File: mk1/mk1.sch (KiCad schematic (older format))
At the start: 121 parts, among them U1 STM32F070CBTx

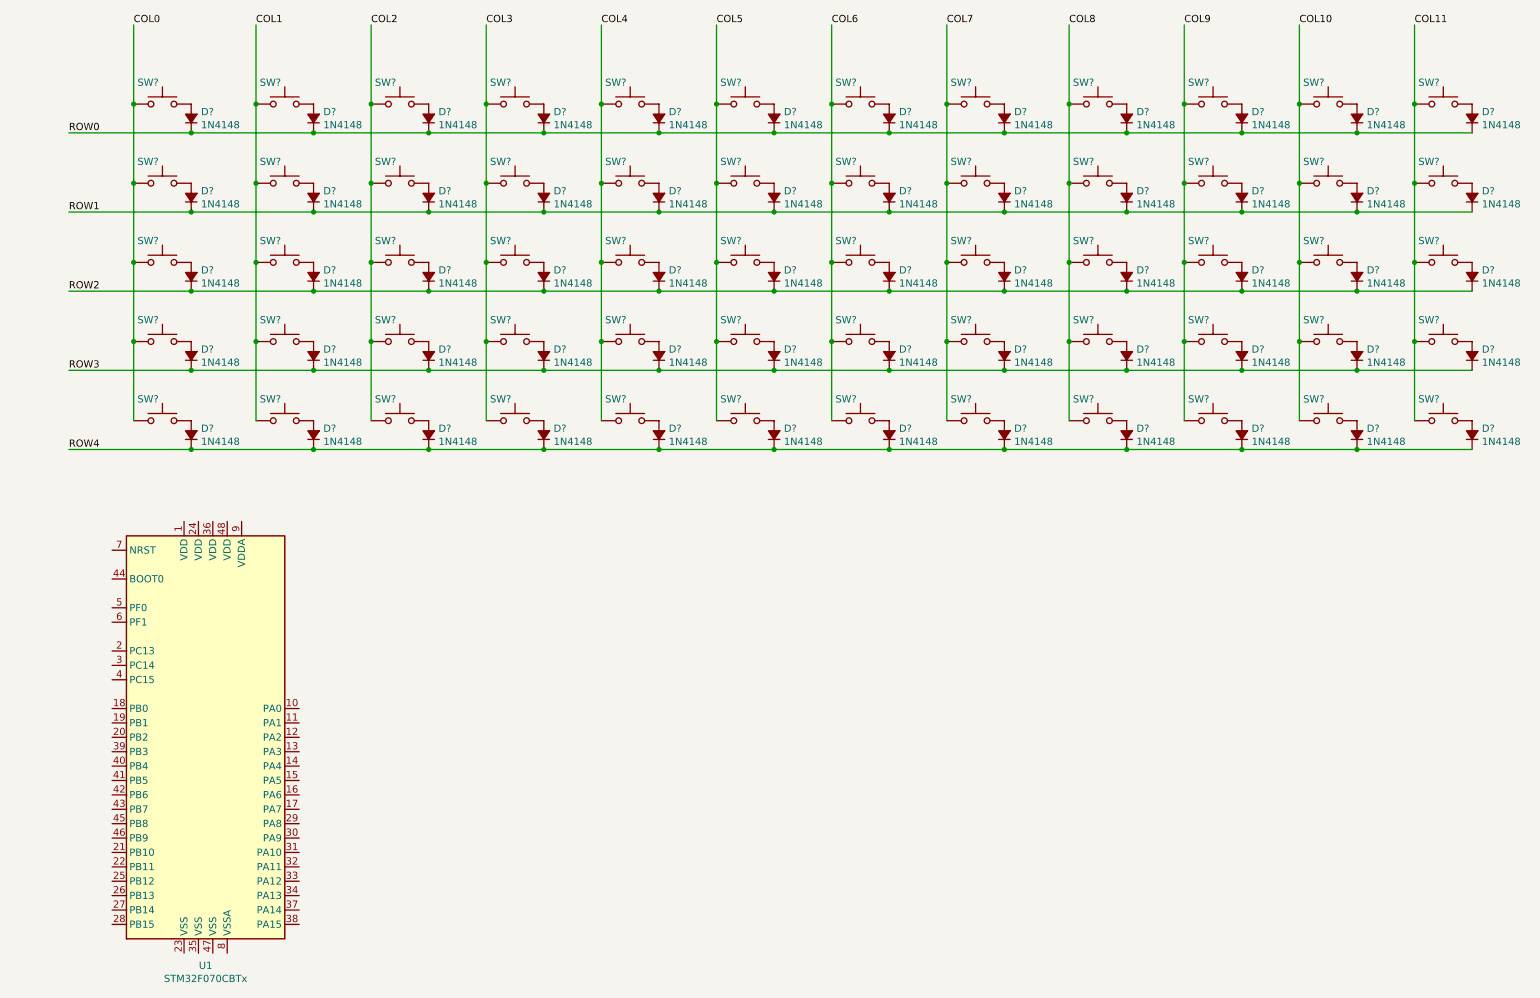
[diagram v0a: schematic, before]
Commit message: using ML switch built i jumper bar
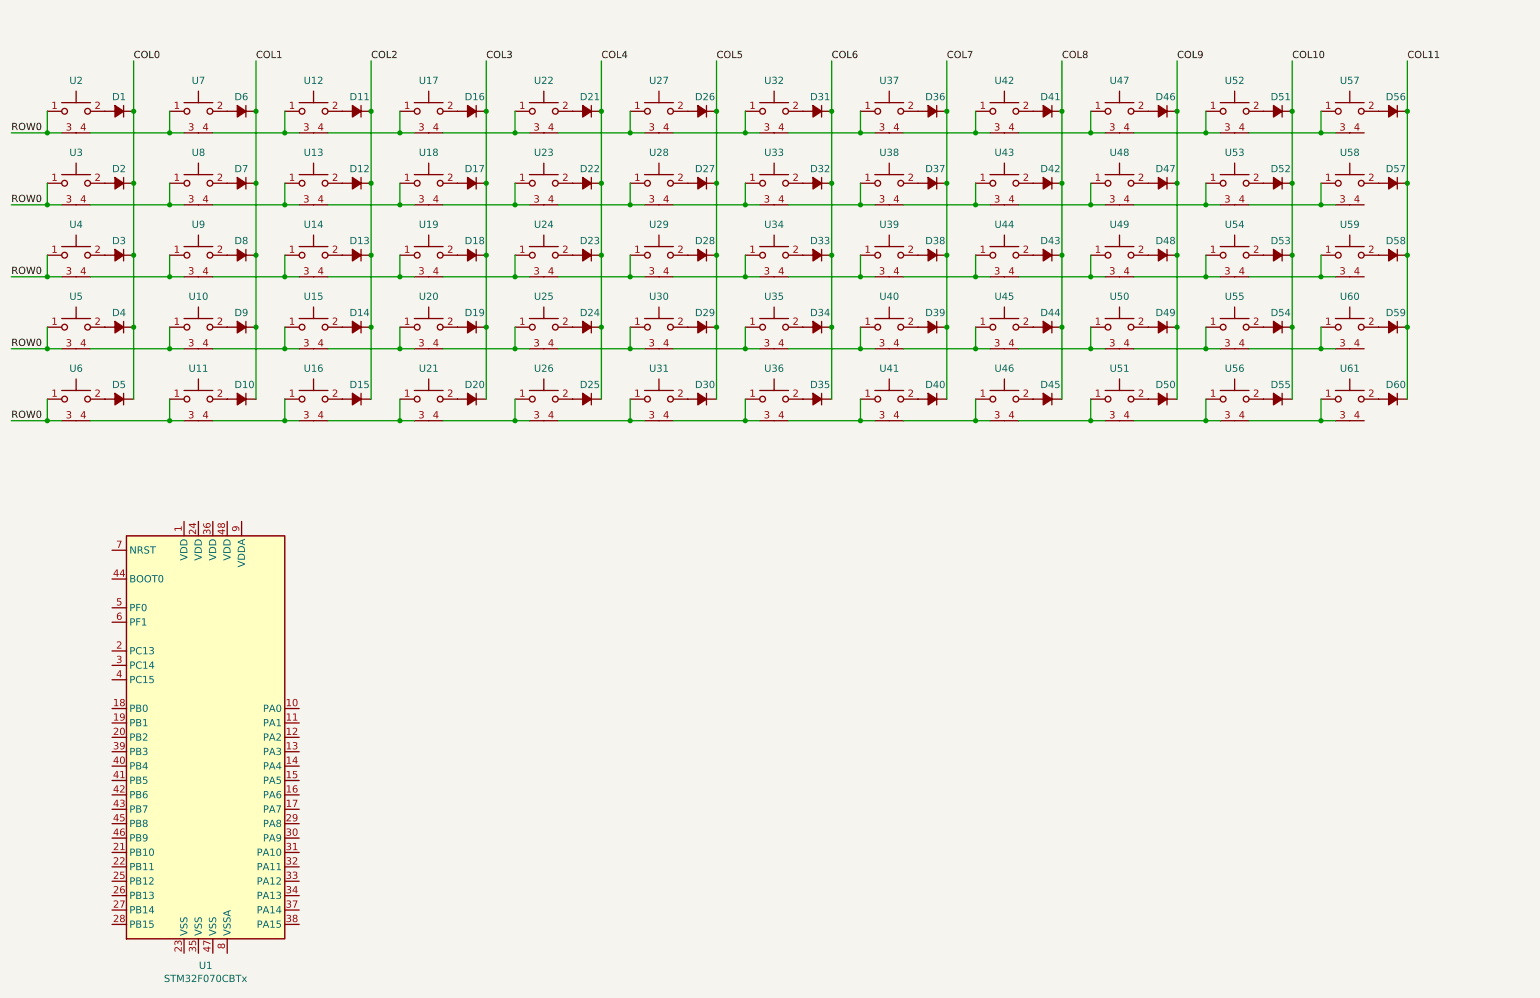
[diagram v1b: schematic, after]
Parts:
- removed D? (x59): 1N4148, symbol Device:D_Small_ALT
- removed SW? (x60): SW_Push, symbol Switch:SW_Push
- added D10, D11, D12, D13, D14, D15, D16, D17, D18, D19, D2, D20, D21, D22, D23, D24, D25, D26, D27, D28, D29, D3, D30, D31, D32, D33, D34, D35, D36, D37, D38, D39, D4, D40, D41, D42, D43, D44, D45, D46, D47, D48, D49, D5, D50, D51, D52, D53, D54, D55, D56, D57, D58, D59, D6, D60, D7, D8, D9: 1N4148, Diode_SMD:D_SOD-123, symbol Device:D_Small_ALT
- added U10, U11, U12, U13, U14, U15, U16, U17, U18, U19, U2, U20, U21, U22, U23, U24, U25, U26, U27, U28, U29, U3, U30, U31, U32, U33, U34, U35, U36, U37, U38, U39, U4, U40, U41, U42, U43, U44, U45, U46, U47, U48, U49, U5, U50, U51, U52, U53, U54, U55, U56, U57, U58, U59, U6, U60, U61, U7, U8, U9: CHERRY_ML, Switches:CHERRY_ML, symbol keyswitch:CHERRY_ML
- D1: renamed from D?; footprint (none) -> Diode_SMD:D_SOD-123
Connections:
- net COL0: now also D1.1 (K), D2.1 (K), D3.1 (K), D4.1 (K), D5.1 (K)
- net COL1: now also D10.1 (K), D6.1 (K), D7.1 (K), D8.1 (K), D9.1 (K)
- net COL10: now also D51.1 (K), D52.1 (K), D53.1 (K), D54.1 (K), D55.1 (K)
- net COL11: now also D56.1 (K), D57.1 (K), D58.1 (K), D59.1 (K), D60.1 (K)
- net COL2: now also D11.1 (K), D12.1 (K), D13.1 (K), D14.1 (K), D15.1 (K)
- net COL3: now also D16.1 (K), D17.1 (K), D18.1 (K), D19.1 (K), D20.1 (K)
- net COL4: now also D21.1 (K), D22.1 (K), D23.1 (K), D24.1 (K), D25.1 (K)
- net COL5: now also D26.1 (K), D27.1 (K), D28.1 (K), D29.1 (K), D30.1 (K)
- net COL6: now also D31.1 (K), D32.1 (K), D33.1 (K), D34.1 (K), D35.1 (K)
- net COL7: now also D36.1 (K), D37.1 (K), D38.1 (K), D39.1 (K), D40.1 (K)
- net COL8: now also D41.1 (K), D42.1 (K), D43.1 (K), D44.1 (K), D45.1 (K)
- net COL9: now also D46.1 (K), D47.1 (K), D48.1 (K), D49.1 (K), D50.1 (K)
- net ROW0: now also U2.1, U2.3, U3.1, U3.3, U4.1, U4.3, U5.1, U5.3, U6.1, U6.3; no longer D1.1 (K)
- net at D1.2 (A): now also U2.2
- new net: U2.4, U7.1, U7.3
- new net: D6.2 (A), U7.2
- new net: U12.1, U12.3, U7.4
- new net: D11.2 (A), U12.2
- new net: U12.4, U17.1, U17.3
- new net: D16.2 (A), U17.2
- new net: U17.4, U22.1, U22.3
- new net: D21.2 (A), U22.2
- new net: U22.4, U27.1, U27.3
- new net: D26.2 (A), U27.2
- new net: U27.4, U32.1, U32.3
- new net: D31.2 (A), U32.2
- new net: U32.4, U37.1, U37.3
- new net: D36.2 (A), U37.2
- new net: U37.4, U42.1, U42.3
- new net: D41.2 (A), U42.2
- new net: U42.4, U47.1, U47.3
- new net: D46.2 (A), U47.2
- new net: U47.4, U52.1, U52.3
- new net: D51.2 (A), U52.2
- new net: U52.4, U57.1, U57.3
- new net: D56.2 (A), U57.2
- new net: D2.2 (A), U3.2
- new net: U3.4, U8.1, U8.3
- new net: D7.2 (A), U8.2
- new net: U13.1, U13.3, U8.4
- new net: D12.2 (A), U13.2
- new net: U13.4, U18.1, U18.3
- new net: D17.2 (A), U18.2
- new net: U18.4, U23.1, U23.3
- new net: D22.2 (A), U23.2
- new net: U23.4, U28.1, U28.3
- new net: D27.2 (A), U28.2
- new net: U28.4, U33.1, U33.3
- new net: D32.2 (A), U33.2
- new net: U33.4, U38.1, U38.3
- new net: D37.2 (A), U38.2
- new net: U38.4, U43.1, U43.3
- new net: D42.2 (A), U43.2
- new net: U43.4, U48.1, U48.3
- new net: D47.2 (A), U48.2
- new net: U48.4, U53.1, U53.3
- new net: D52.2 (A), U53.2
- new net: U53.4, U58.1, U58.3
- new net: D57.2 (A), U58.2
- new net: D3.2 (A), U4.2
- new net: U4.4, U9.1, U9.3
- new net: D8.2 (A), U9.2
- new net: U14.1, U14.3, U9.4
- new net: D13.2 (A), U14.2
- new net: U14.4, U19.1, U19.3
- new net: D18.2 (A), U19.2
- new net: U19.4, U24.1, U24.3
- new net: D23.2 (A), U24.2
- new net: U24.4, U29.1, U29.3
- new net: D28.2 (A), U29.2
- new net: U29.4, U34.1, U34.3
- new net: D33.2 (A), U34.2
- new net: U34.4, U39.1, U39.3
- new net: D38.2 (A), U39.2
- new net: U39.4, U44.1, U44.3
- new net: D43.2 (A), U44.2
- new net: U44.4, U49.1, U49.3
- new net: D48.2 (A), U49.2
- new net: U49.4, U54.1, U54.3
- new net: D53.2 (A), U54.2
- new net: U54.4, U59.1, U59.3
- new net: D58.2 (A), U59.2
- new net: D4.2 (A), U5.2
- new net: U10.1, U10.3, U5.4
- new net: D9.2 (A), U10.2
- new net: U10.4, U15.1, U15.3
- new net: D14.2 (A), U15.2
- new net: U15.4, U20.1, U20.3
- new net: D19.2 (A), U20.2
- new net: U20.4, U25.1, U25.3
- new net: D24.2 (A), U25.2
- new net: U25.4, U30.1, U30.3
- new net: D29.2 (A), U30.2
- new net: U30.4, U35.1, U35.3
- new net: D34.2 (A), U35.2
- new net: U35.4, U40.1, U40.3
- new net: D39.2 (A), U40.2
- new net: U40.4, U45.1, U45.3
- new net: D44.2 (A), U45.2
- new net: U45.4, U50.1, U50.3
- new net: D49.2 (A), U50.2
- new net: U50.4, U55.1, U55.3
- new net: D54.2 (A), U55.2
- new net: U55.4, U60.1, U60.3
- new net: D59.2 (A), U60.2
- new net: D5.2 (A), U6.2
- new net: U11.1, U11.3, U6.4
- new net: D10.2 (A), U11.2
- new net: U11.4, U16.1, U16.3
- new net: D15.2 (A), U16.2
- new net: U16.4, U21.1, U21.3
- new net: D20.2 (A), U21.2
- new net: U21.4, U26.1, U26.3
- new net: D25.2 (A), U26.2
- new net: U26.4, U31.1, U31.3
- new net: D30.2 (A), U31.2
- new net: U31.4, U36.1, U36.3
- new net: D35.2 (A), U36.2
- new net: U36.4, U41.1, U41.3
- new net: D40.2 (A), U41.2
- new net: U41.4, U46.1, U46.3
- new net: D45.2 (A), U46.2
- new net: U46.4, U51.1, U51.3
- new net: D50.2 (A), U51.2
- new net: U51.4, U56.1, U56.3
- new net: D55.2 (A), U56.2
- new net: U56.4, U61.1, U61.3
- new net: D60.2 (A), U61.2
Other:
- moved on the sheet: D1
